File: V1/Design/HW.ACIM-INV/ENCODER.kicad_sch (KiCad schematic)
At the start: 21 parts, among them J8 ENCODER, Q2 60V/265mA, Q7 60V/265mA, Q8 60V/265mA, Q9 60V/265mA

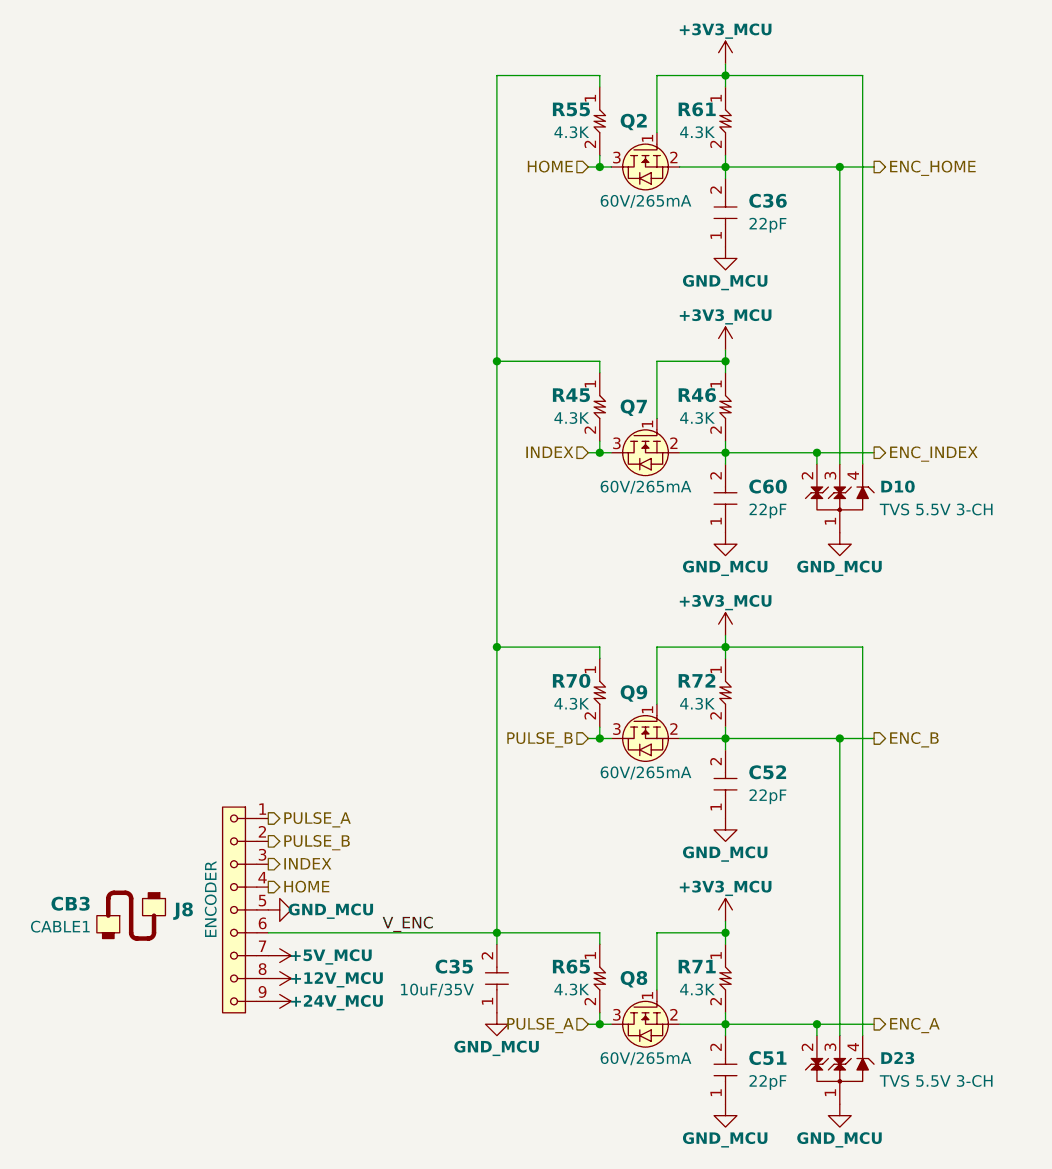
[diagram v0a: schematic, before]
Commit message: V1 schematic update 16
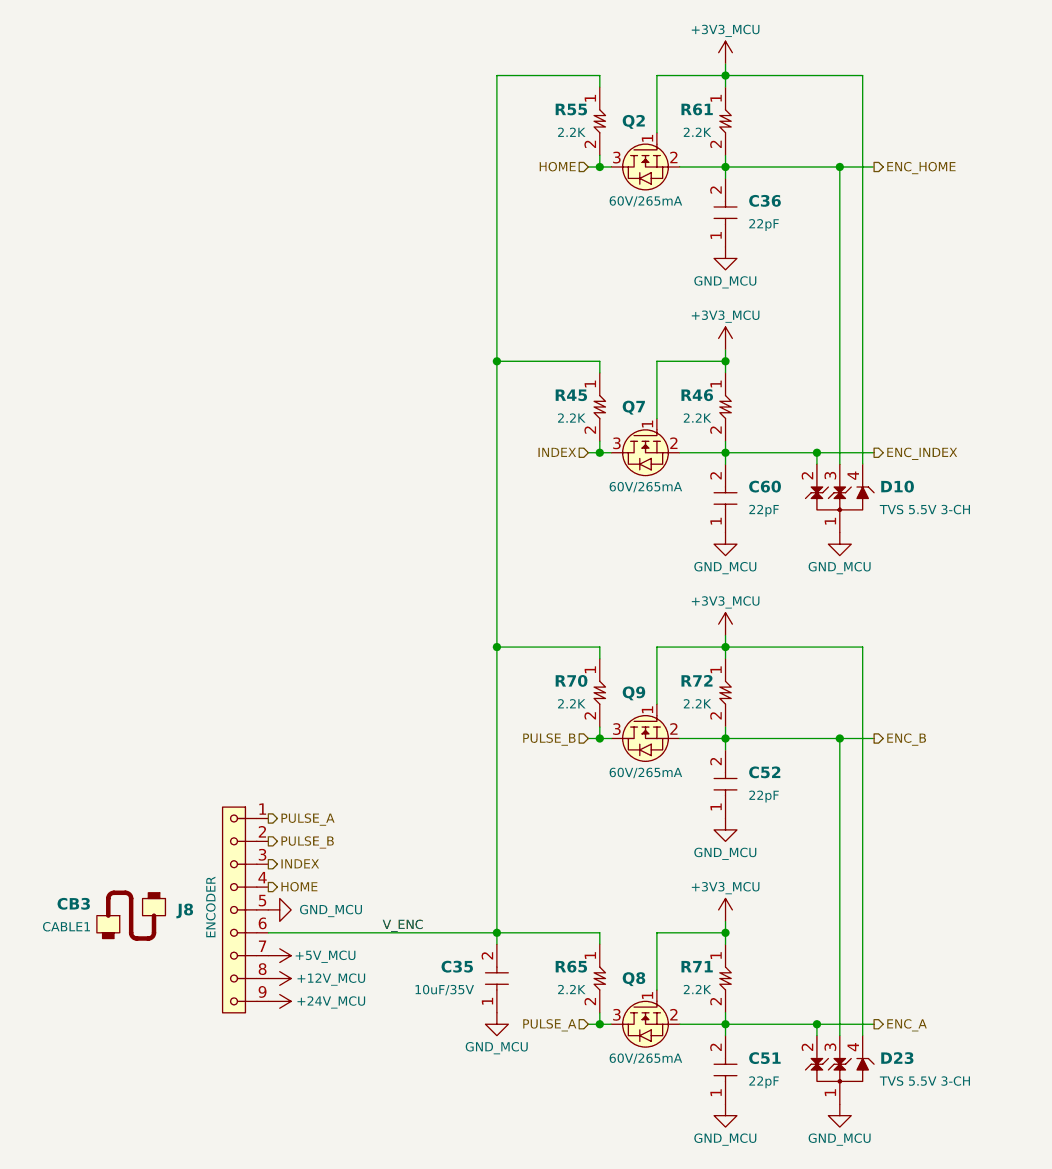
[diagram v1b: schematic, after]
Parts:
- C35: footprint SAMPI:CAP0603 -> SAMPI:CAP1206; MFT Samsung -> (none); MNP CL10A106MQ8NNNC -> (none)
- R45, R46, R55, R61, R65, R70, R71, R72: value 4.3K -> 2.2K; MFT YAGEO -> (none); MNP AC0603FR-074K3L -> (none)
